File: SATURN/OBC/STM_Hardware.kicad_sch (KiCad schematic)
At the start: 24 parts, among them IC1 STM32H735AGI6, J1 SWD Pins, J2 USB_C_Receptacle

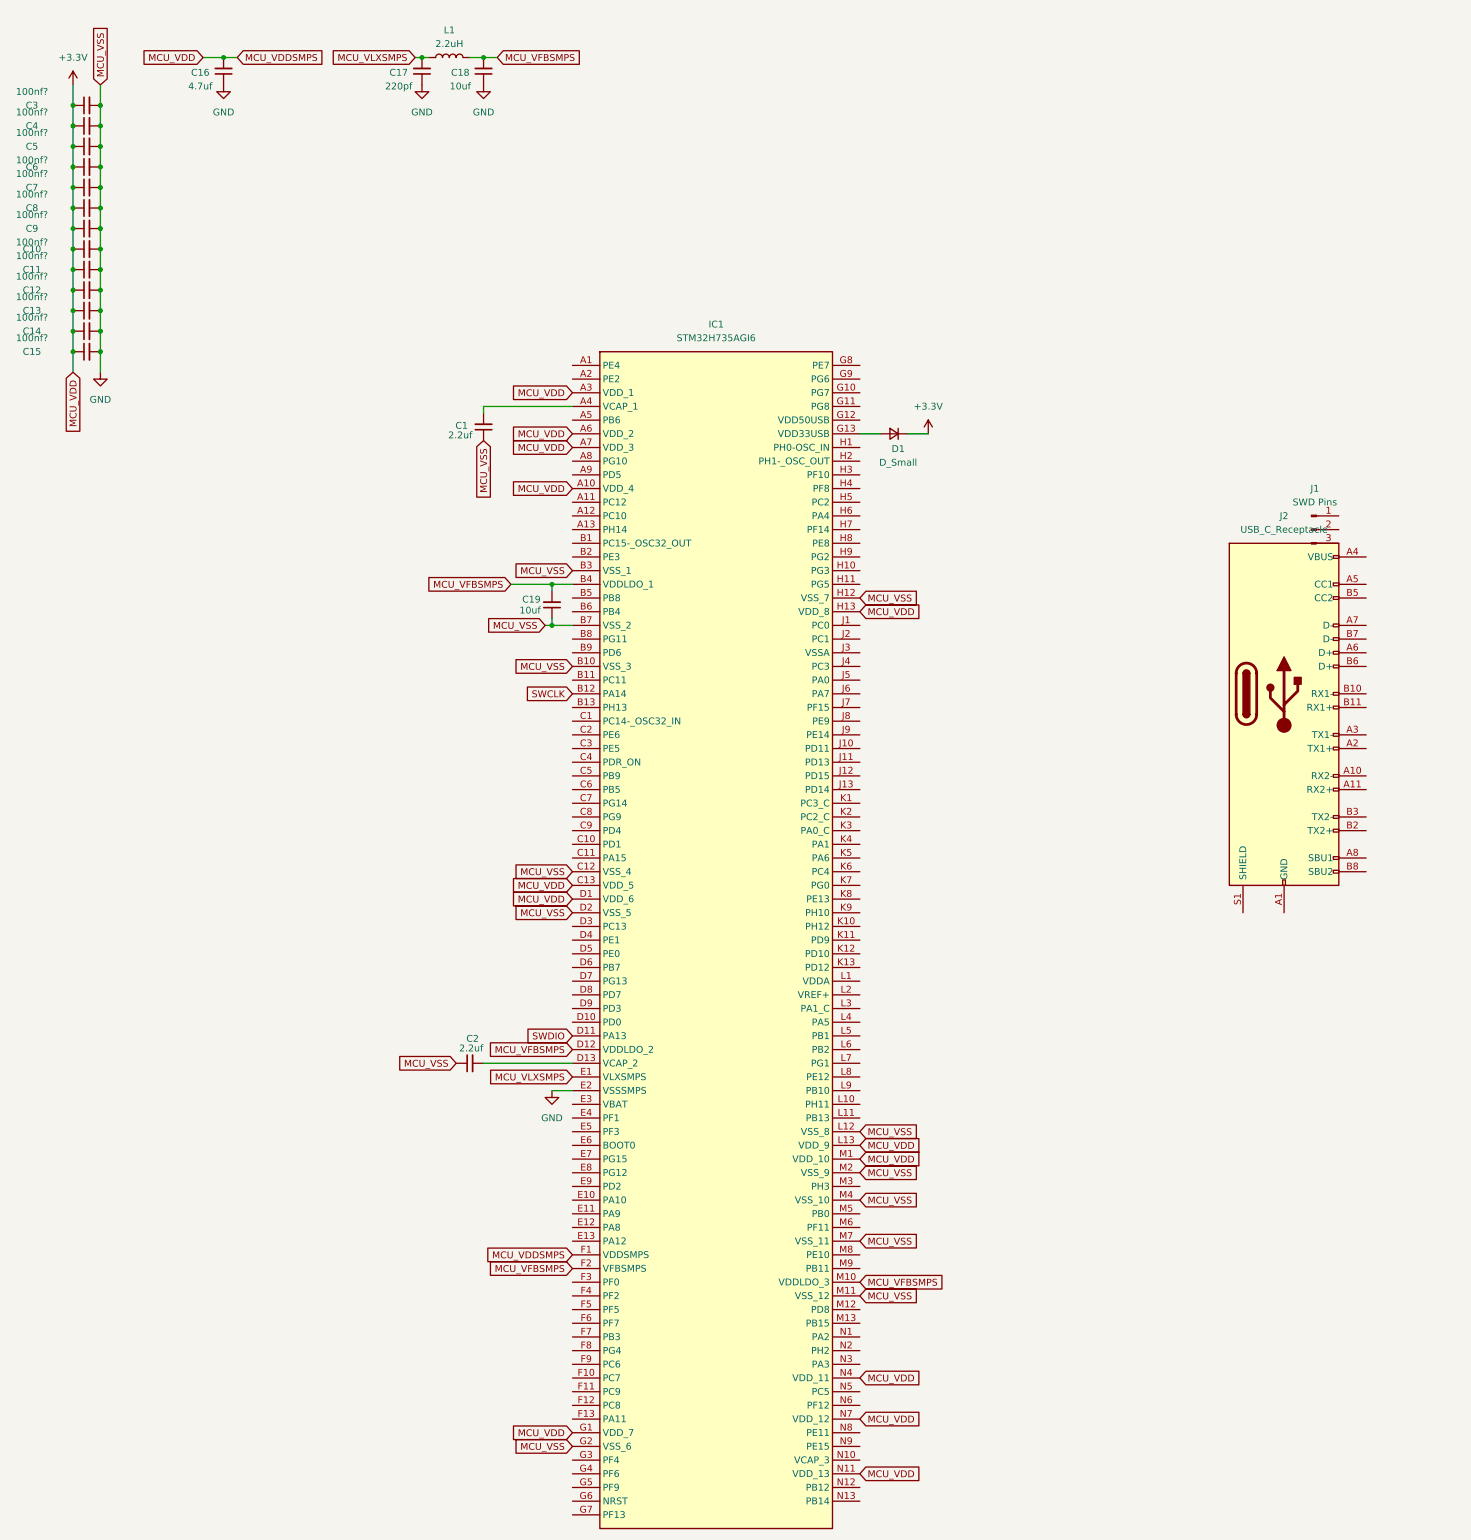
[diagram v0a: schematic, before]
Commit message: Messy but working on turing it into a hierarchical schematic
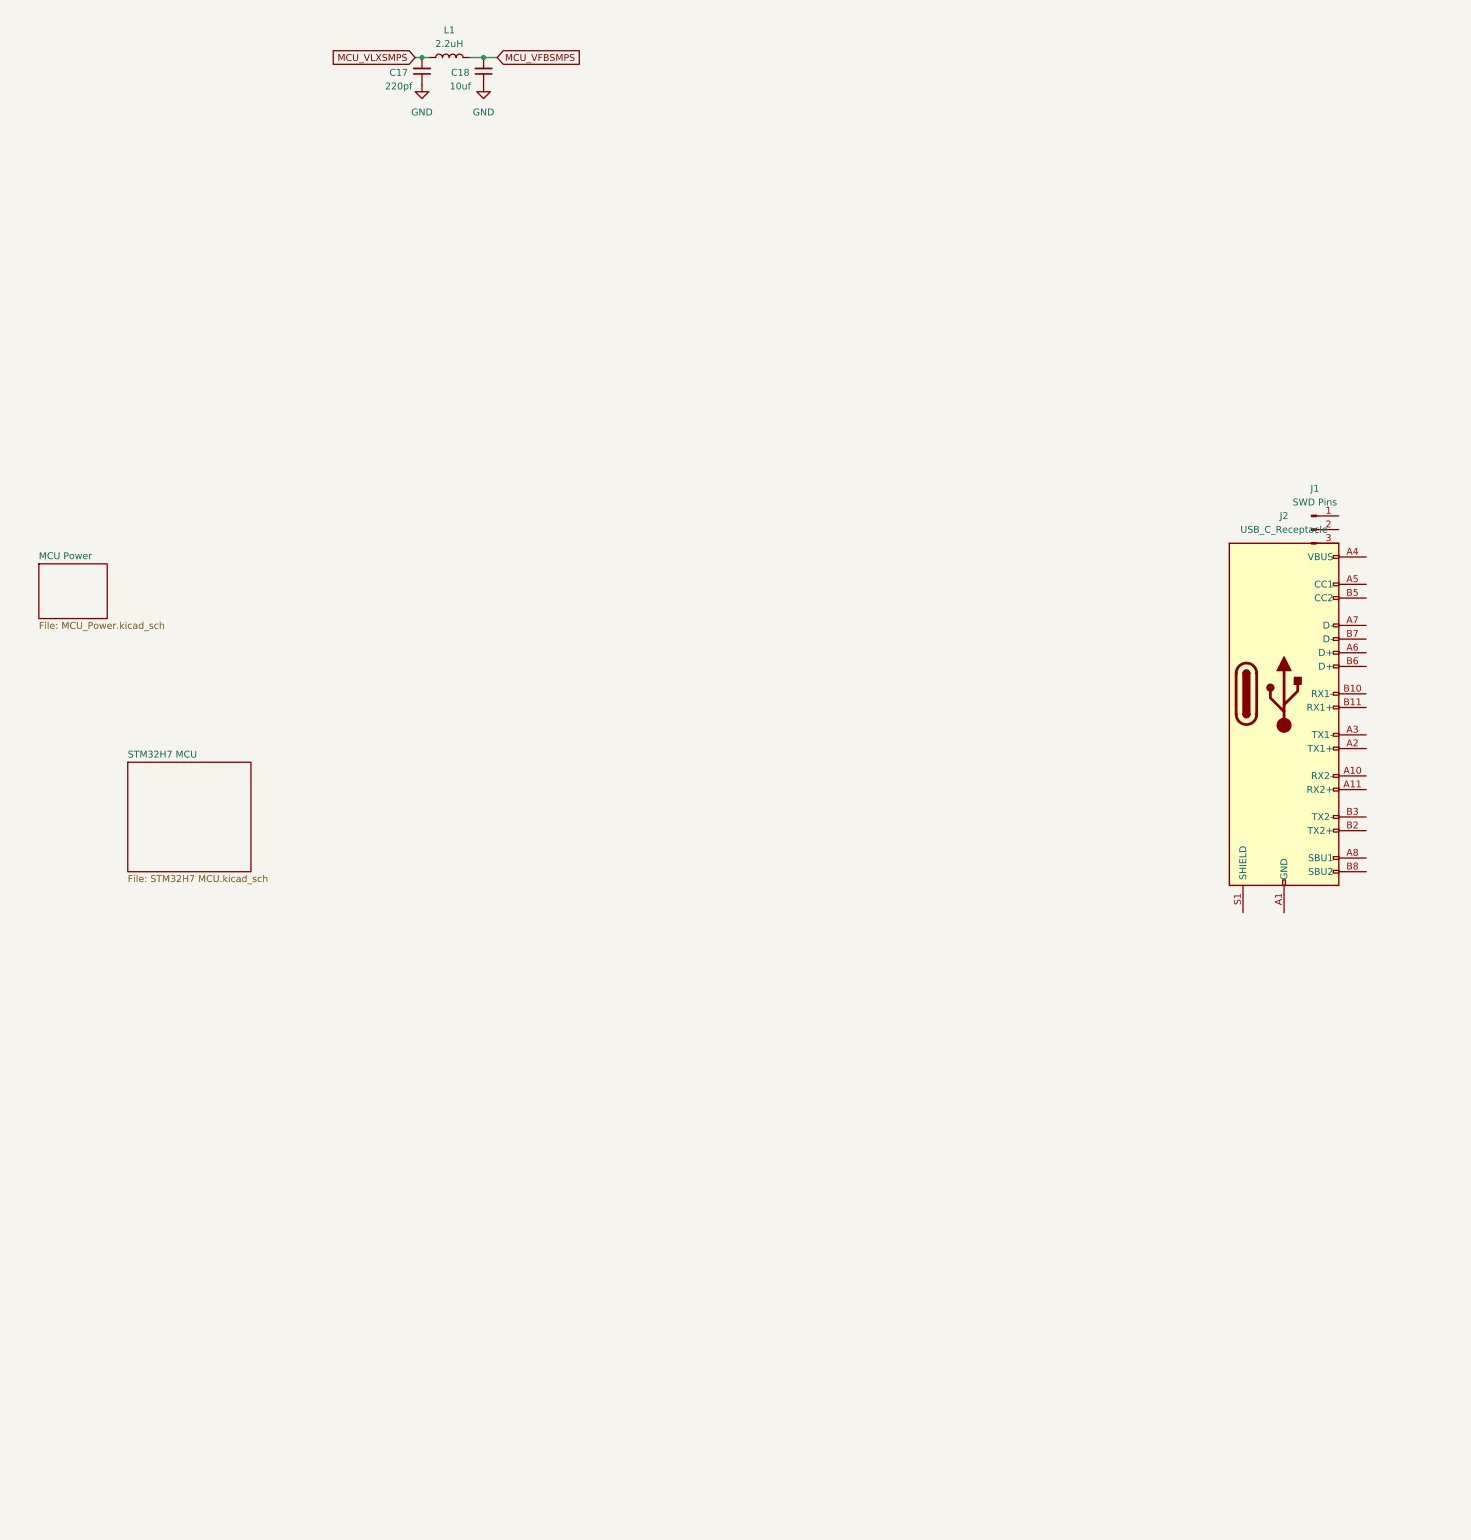
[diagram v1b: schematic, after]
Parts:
- removed C1, C2: 2.2uf, Capacitor_SMD:C_0603_1608Metric, symbol Device:C_Small
- removed C10, C11, C12, C13, C14, C15, C3, C4, C5, C6, C7, C8, C9: 100nf?, Capacitor_SMD:C_0603_1608Metric, symbol Device:C_Small
- removed C16: 4.7uf, Capacitor_SMD:C_0603_1608Metric, symbol Device:C_Small
- removed C19: 10uf, Capacitor_SMD:C_0603_1608Metric, symbol Device:C_Small
- removed D1: D_Small, symbol Device:D_Small
- removed IC1: STM32H735AGI6, Gabriel_footprints:BGA169C50P13X13_700X700X60, symbol STM32H735AGI6:STM32H735AGI6
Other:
- added sheet MCU Power (MCU_Power.kicad_sch)
- added sheet STM32H7 MCU (STM32H7 MCU.kicad_sch)

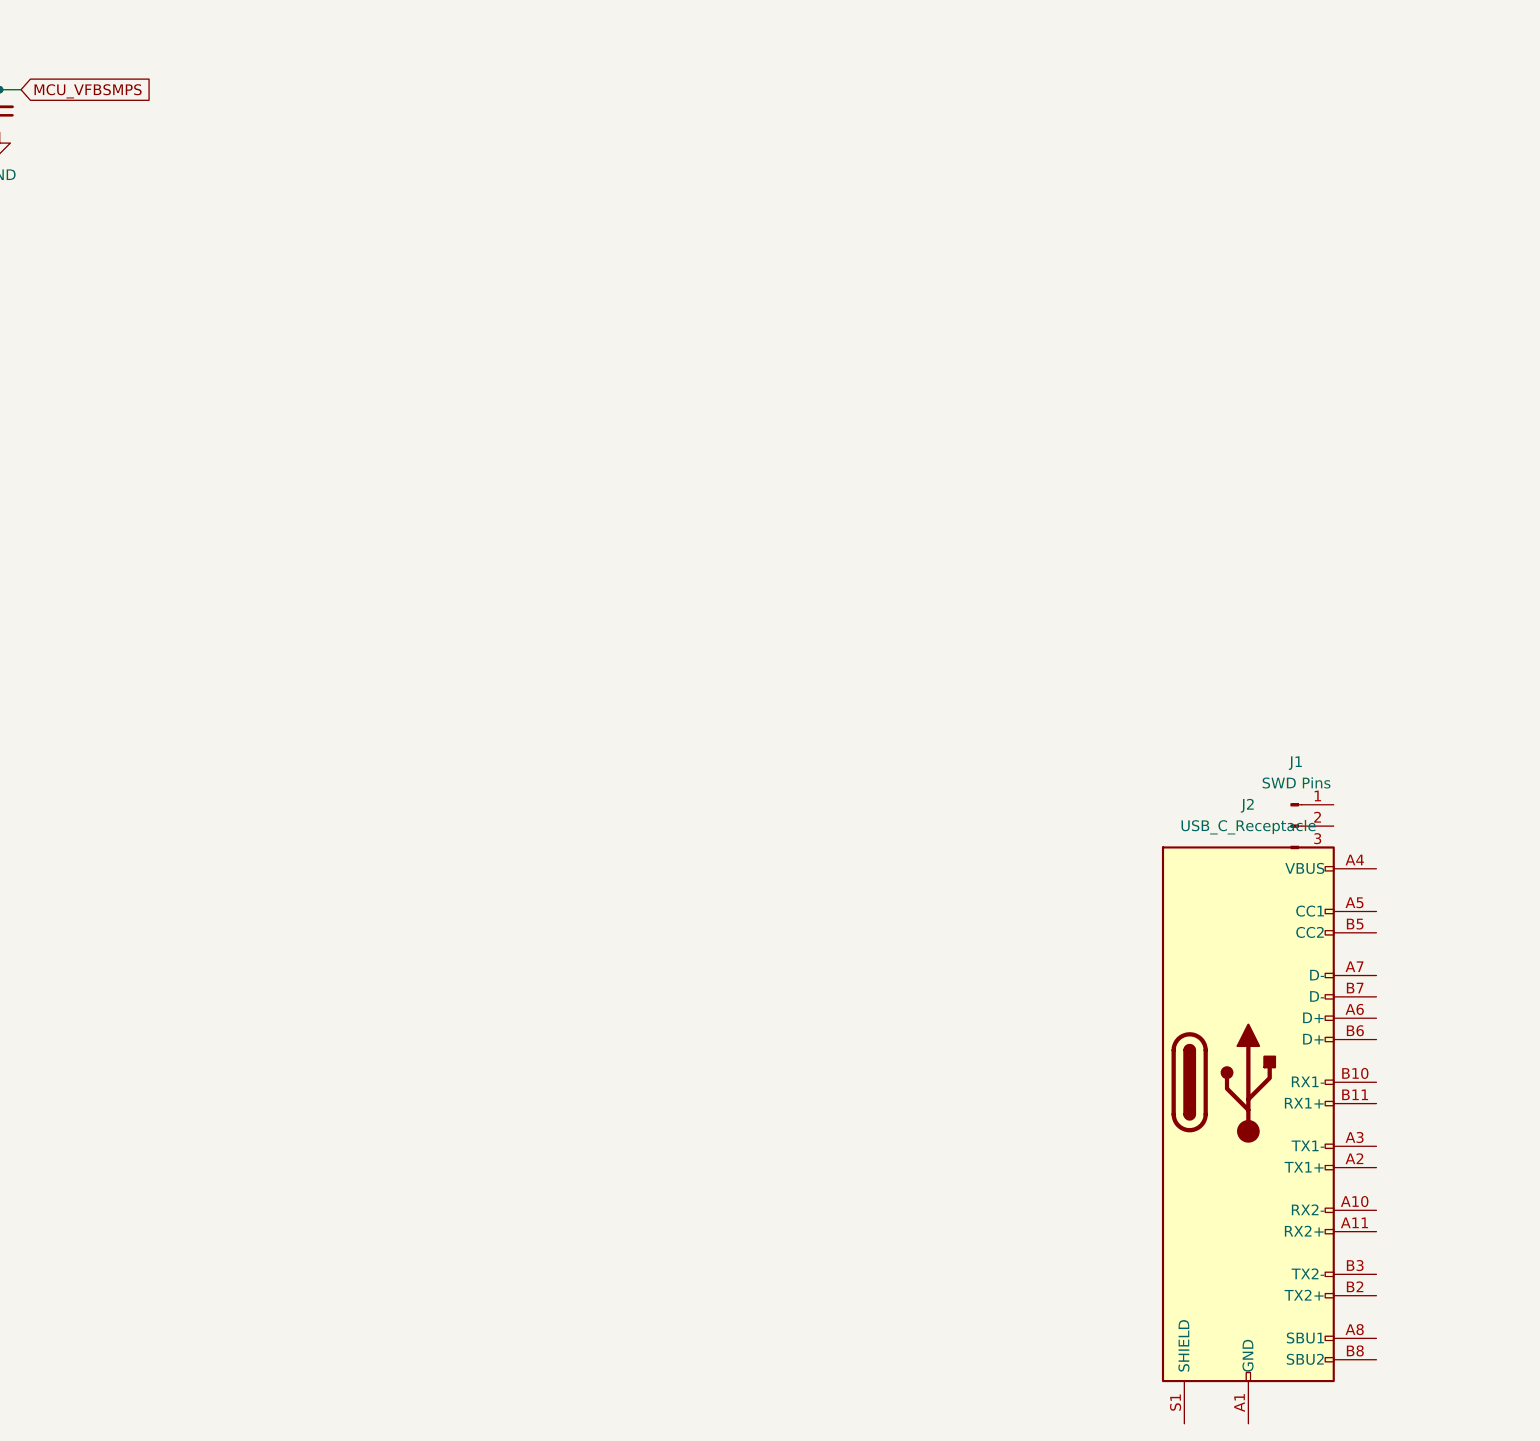
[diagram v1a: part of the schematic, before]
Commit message: usb
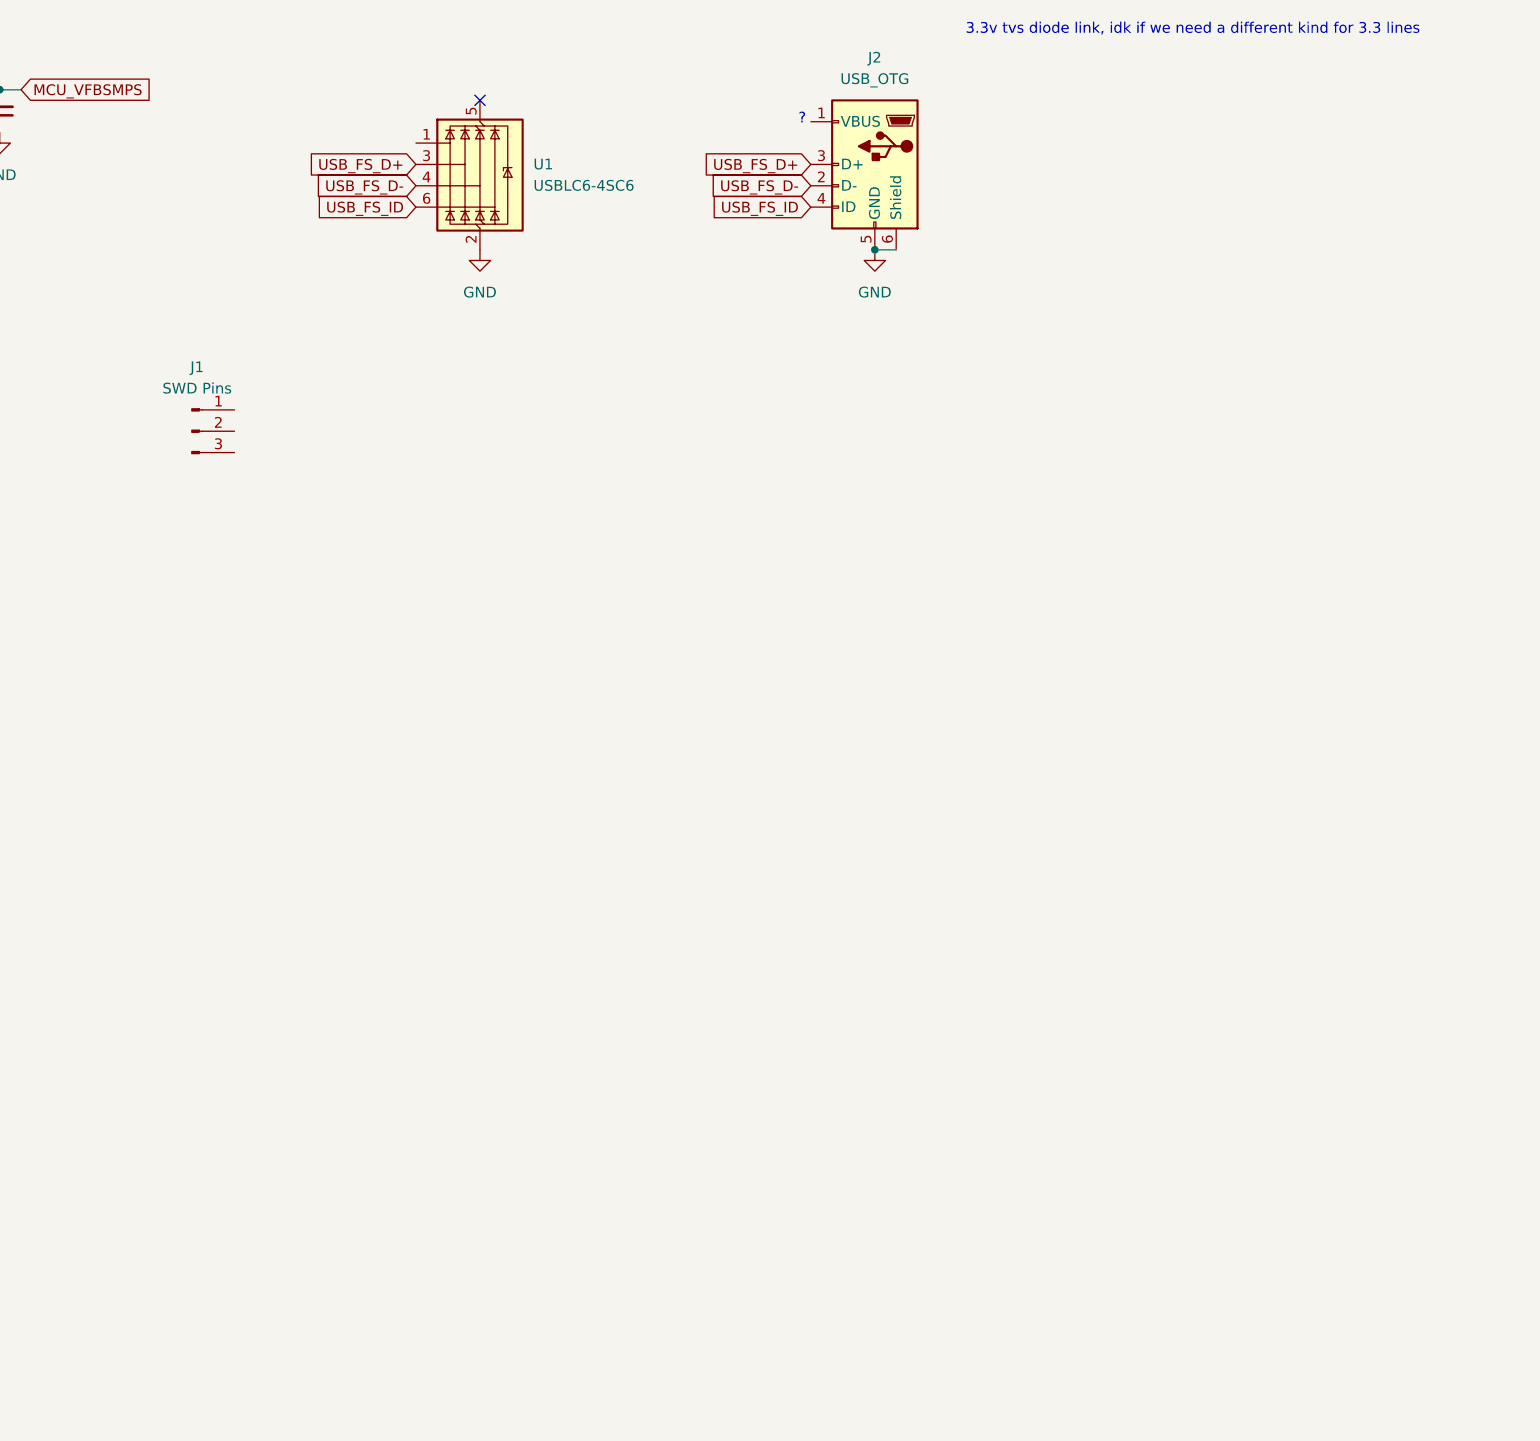
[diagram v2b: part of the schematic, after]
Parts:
- removed J2: USB_C_Receptacle, symbol Connector:USB_C_Receptacle
- added J2: USB_OTG, symbol Connector:USB_OTG
- added U1: USBLC6-4SC6, Package_TO_SOT_SMD:SOT-23-6, symbol Power_Protection:USBLC6-4SC6
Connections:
- net GND: now also J2.5 (GND), J2.6 (Shield), U1.2 (GND)
- new net USB_FS_D+: J2.3 (D+), U1.3 (I/O2)
- new net USB_FS_D-: J2.2 (D-), U1.4 (I/O3)
- new net USB_FS_ID: J2.4 (ID), U1.6 (I/O4)
- no-connect marks 0 -> 1
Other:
- note added: "3.3v tvs diode link, idk if we need a different kind for 3.3 lines"
- note added: "?"
- moved on the sheet: J1
